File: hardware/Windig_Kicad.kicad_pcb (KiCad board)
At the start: 2 copper layers, 86.4 x 49.5 mm, 31 parts, among them J1 Barrel_Jack, J10 USB_B, J11 Conn_02x03, J2 Conn_01x04, J3 Conn_01x04, J4 Conn_01x04, J5 Conn_01x04, J6 Conn_01x04, J7 Conn_01x04, J8 Conn_01x04, J9 Conn_01x04, SW1 SW_SPDT, SW2 SW_SPDT, U1 ATmega328P-PU, X1 16Mhz

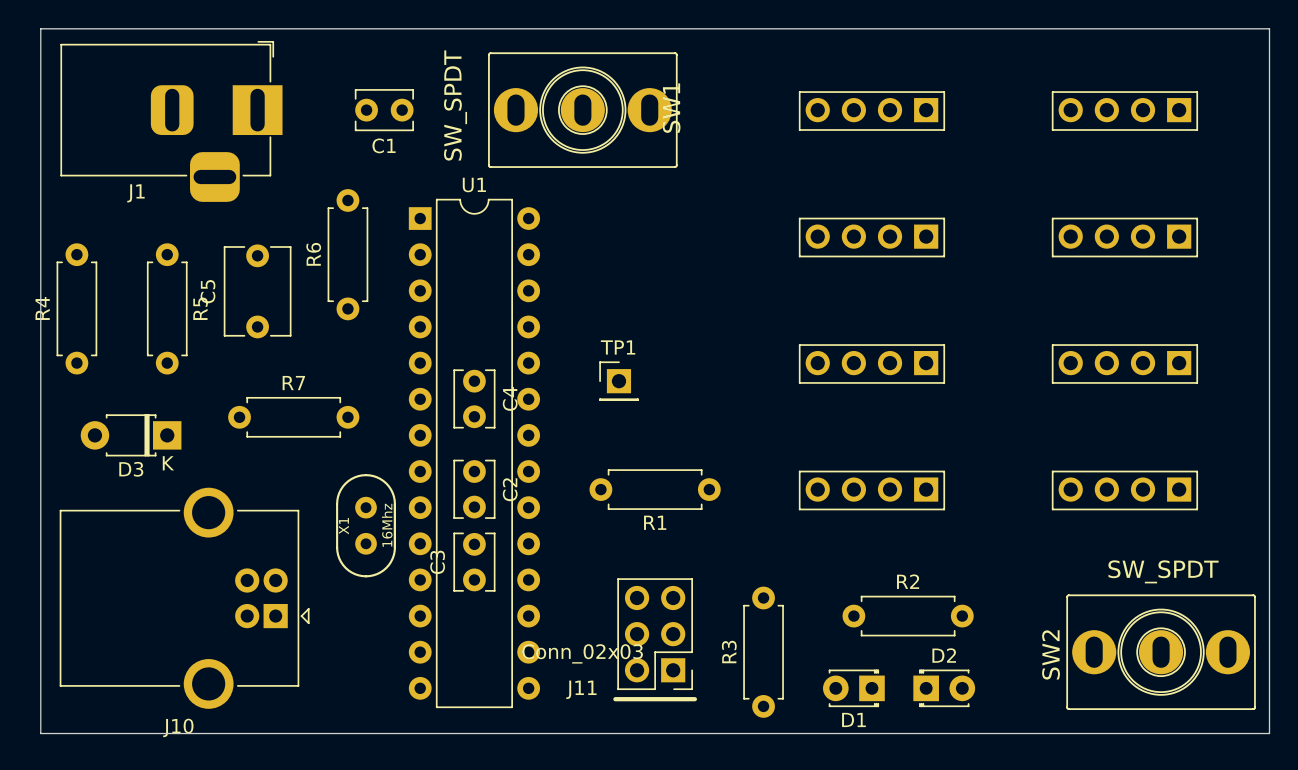
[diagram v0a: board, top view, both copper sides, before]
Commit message: Rough component placemunt update
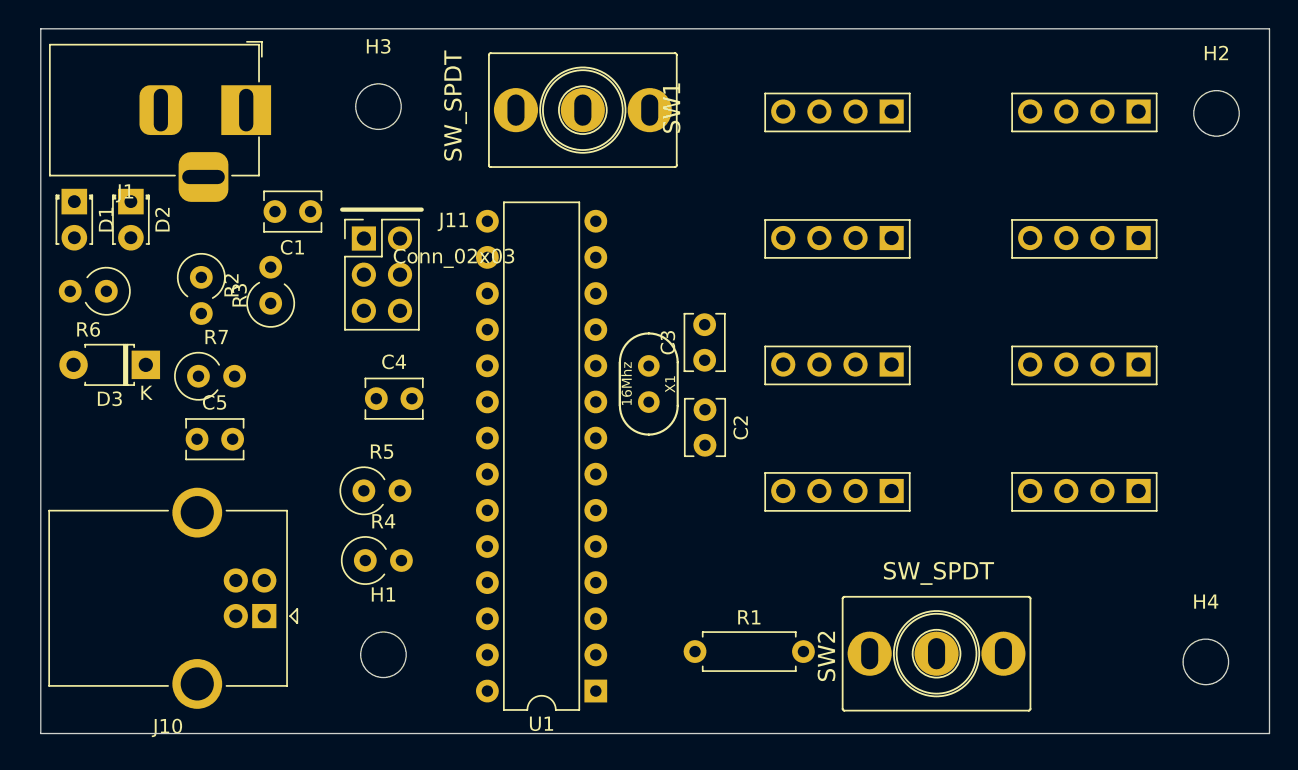
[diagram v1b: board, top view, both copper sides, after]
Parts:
- removed TP1: RESET, Connector_PinHeader_2.54mm:PinHeader_1x01_P2.54mm_Vertical
- added H1: MountingHole, MountingHole:MountingHole_3.2mm_M3, F.Cu at (115.5, 93.5)
- added H2: MountingHole, MountingHole:MountingHole_3.2mm_M3, F.Cu at (174.1, 55.5)
- added H3: MountingHole, MountingHole:MountingHole_3.2mm_M3, F.Cu at (115.2, 55.0)
- added H4: MountingHole, MountingHole:MountingHole_3.2mm_M3, F.Cu at (173.3, 94.0)
- C5: footprint Capacitor_THT:C_Disc_D6.0mm_W4.4mm_P5.00mm -> Capacitor_THT:C_Disc_D3.8mm_W2.6mm_P2.50mm
- R2, R3, R4, R5, R6, R7: footprint Resistor_THT:R_Axial_DIN0207_L6.3mm_D2.5mm_P7.62mm_Horizontal -> Resistor_THT:R_Axial_DIN0309_L9.0mm_D3.2mm_P2.54mm_Vertical
- moved D1 65.7 mm to (93.8, 61.7), turned to 270 degrees
- moved D2 65.5 mm to (97.8, 61.7), turned to 270 degrees
- moved R3 49.7 mm to (102.7, 67.0), turned to 270 degrees
- moved R2 46.5 mm to (107.6, 68.8), turned to 90 degrees
- moved J11 37.3 mm to (114.2, 64.3), turned to 180 degrees
- moved U1 35.4 mm to (130.4, 96.1), turned to 180 degrees
- moved R4 24.6 mm to (114.2, 86.9), turned to 0 degrees
- moved C3 22.4 mm to (138.1, 72.8)
- moved X1 22.2 mm to (134.2, 74.5), turned to 90 degrees
- moved R5 21.6 mm to (114.2, 82.0), turned to 0 degrees
- moved R6 17.0 mm to (96.0, 68.0), turned to 180 degrees
- moved C2 16.8 mm to (138.1, 76.3)
- moved SW2 15.8 mm to (154.4, 93.5)
- moved R1 11.4 mm to (137.4, 93.3), turned to 0 degrees
- moved C1 9.61 mm to (110.4, 62.4)
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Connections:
- U1 pad 21: 5v -> Net-(U1-Pad21)
- U1 pad 23: TACH1A -> TACH1B
- U1 pad 24: TACH1B -> TACH1A
